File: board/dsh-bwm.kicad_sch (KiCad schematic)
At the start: 15 parts, among them IC2 MAX485CSA+T, K1 833H-1C-C-24VDC, K2 833H-1C-C-24VDC, K3 833H-1C-C-24VDC, K4 833H-1C-C-24VDC, Q1 IRLB8721PBF, U1 Pico

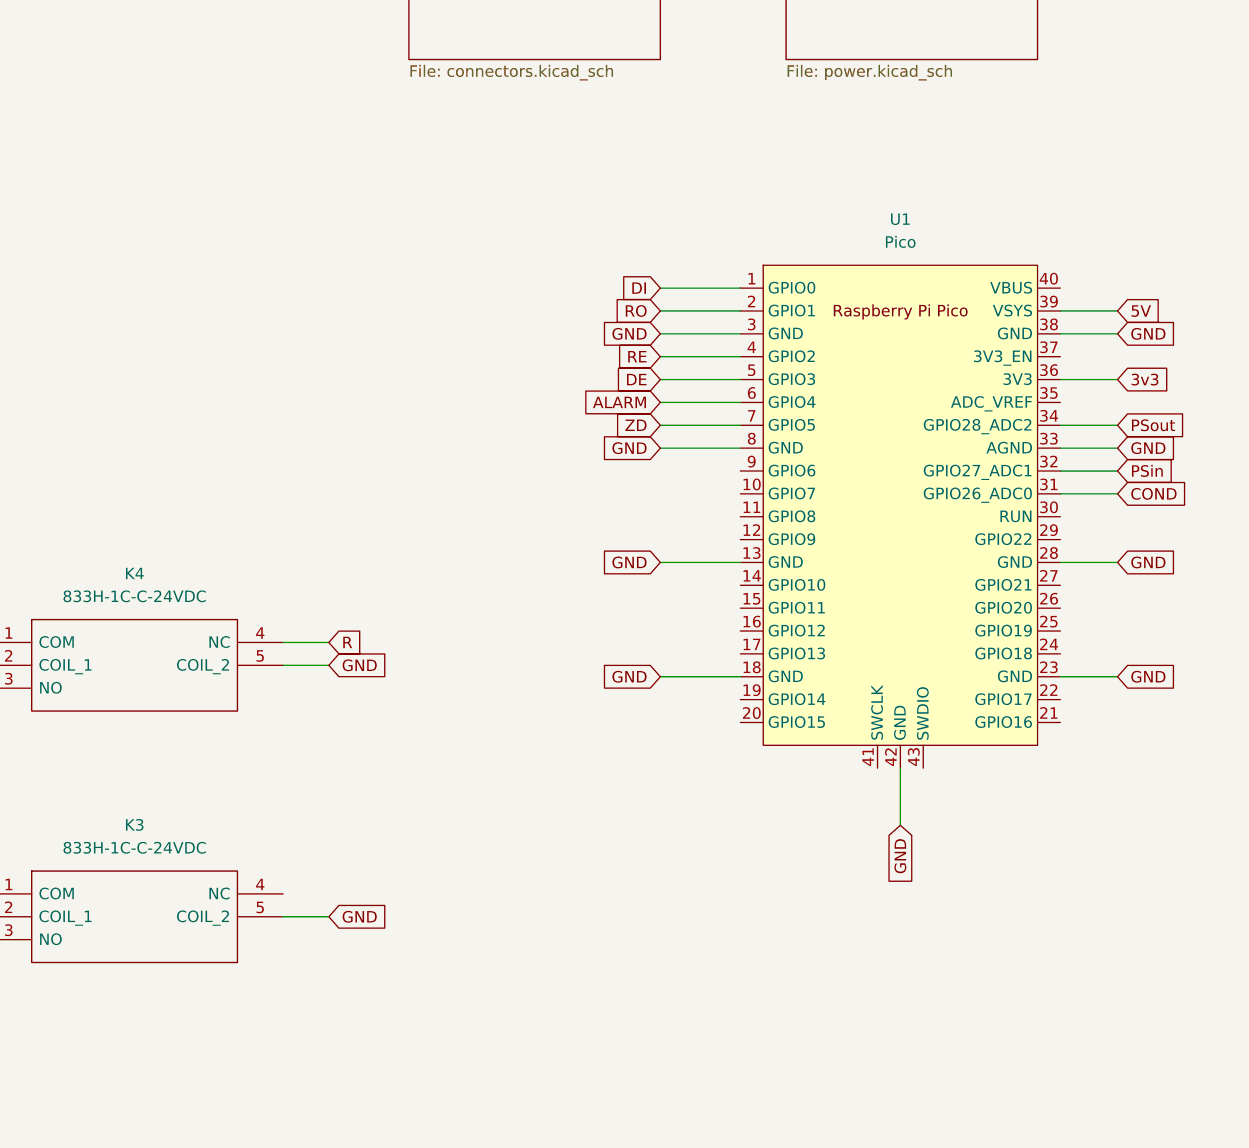
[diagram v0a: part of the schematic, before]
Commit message: RP2040 Stamp
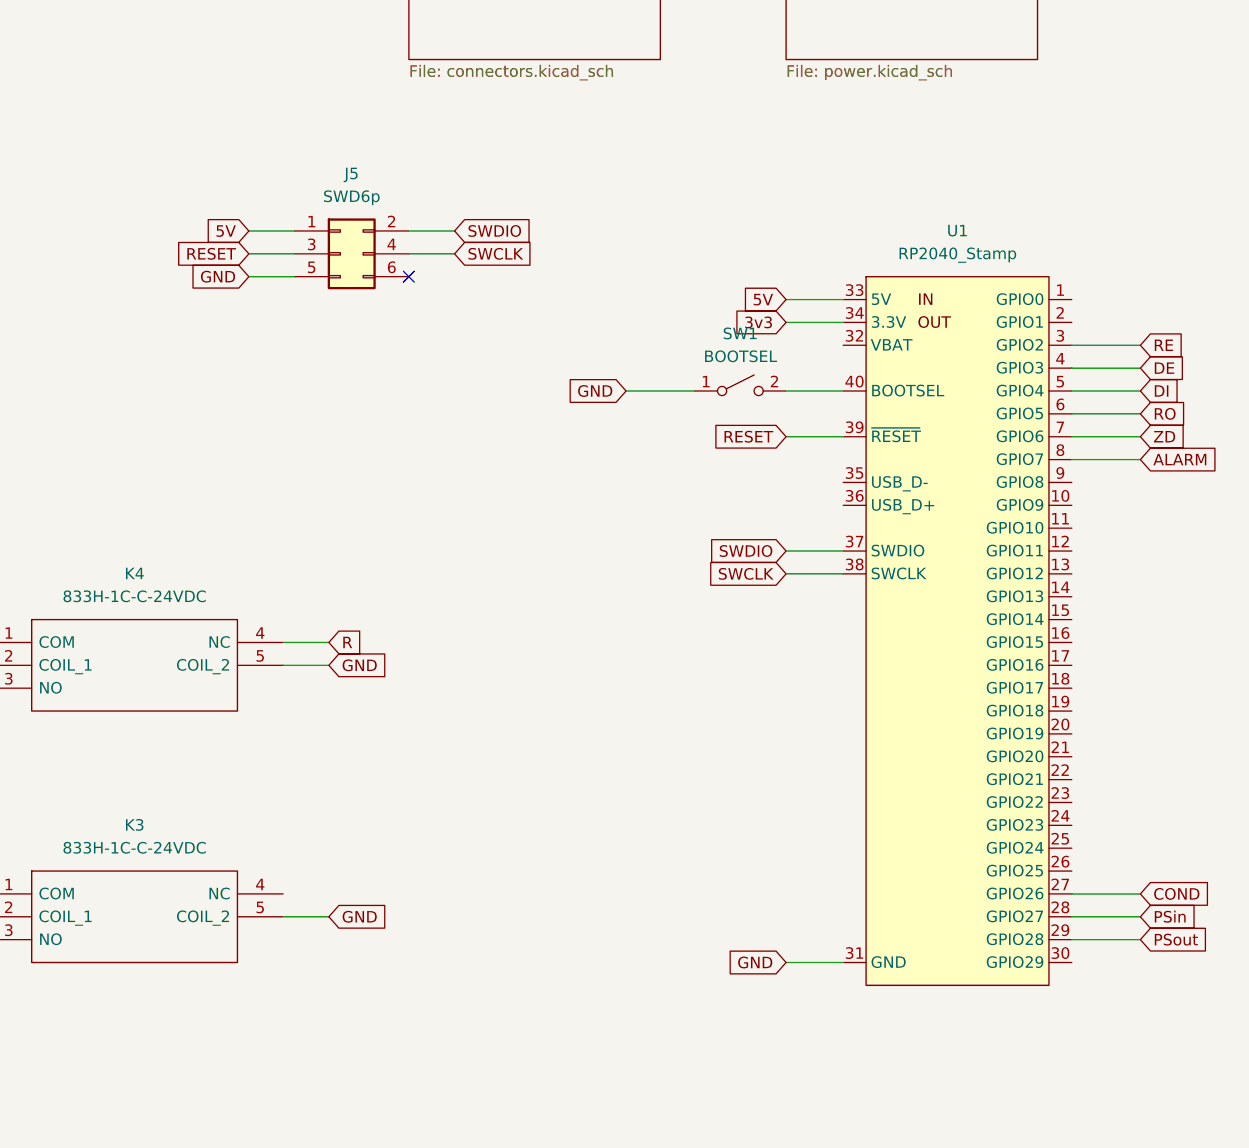
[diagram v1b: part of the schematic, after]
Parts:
- removed U1: Pico, MCU_RaspberryPi_and_Boards:RPi_Pico_SMD_TH, symbol MCU_RaspberryPi_and_Boards:Pico
- added J5: SWD6p, symbol Connector_Generic:Conn_02x03_Odd_Even
- added SW1: BOOTSEL, Button_Switch_SMD:SW_SPST_B3U-1000P, symbol Switch:SW_SPST
- added U1: RP2040_Stamp, SamacSys_Parts:RP2040_Stamp_SMD, symbol RP2040_Stamp:RP2040_Stamp
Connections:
- net 3v3: now also U1.34 (3.3V)
- net 5V: now also J5.1 (Pin_1), U1.33 (5V)
- net ALARM: now also U1.8 (GPIO7)
- net COND: now also U1.27 (GPIO26)
- net DE: now also U1.4 (GPIO3)
- net DI: now also U1.5 (GPIO4)
- net GND: now also J5.5 (Pin_5), SW1.1 (A), U1.31 (GND)
- net PSin: now also U1.28 (GPIO27)
- net PSout: now also U1.29 (GPIO28)
- net RE: now also U1.3 (GPIO2)
- net RO: now also U1.6 (GPIO5)
- net ZD: now also U1.7 (GPIO6)
- new net: SW1.2 (B), U1.40 (BOOTSEL)
- new net RESET: J5.3 (Pin_3), U1.39 (~{RESET})
- new net SWCLK: J5.4 (Pin_4), U1.38 (SWCLK)
- new net SWDIO: J5.2 (Pin_2), U1.37 (SWDIO)
- no-connect marks 0 -> 1

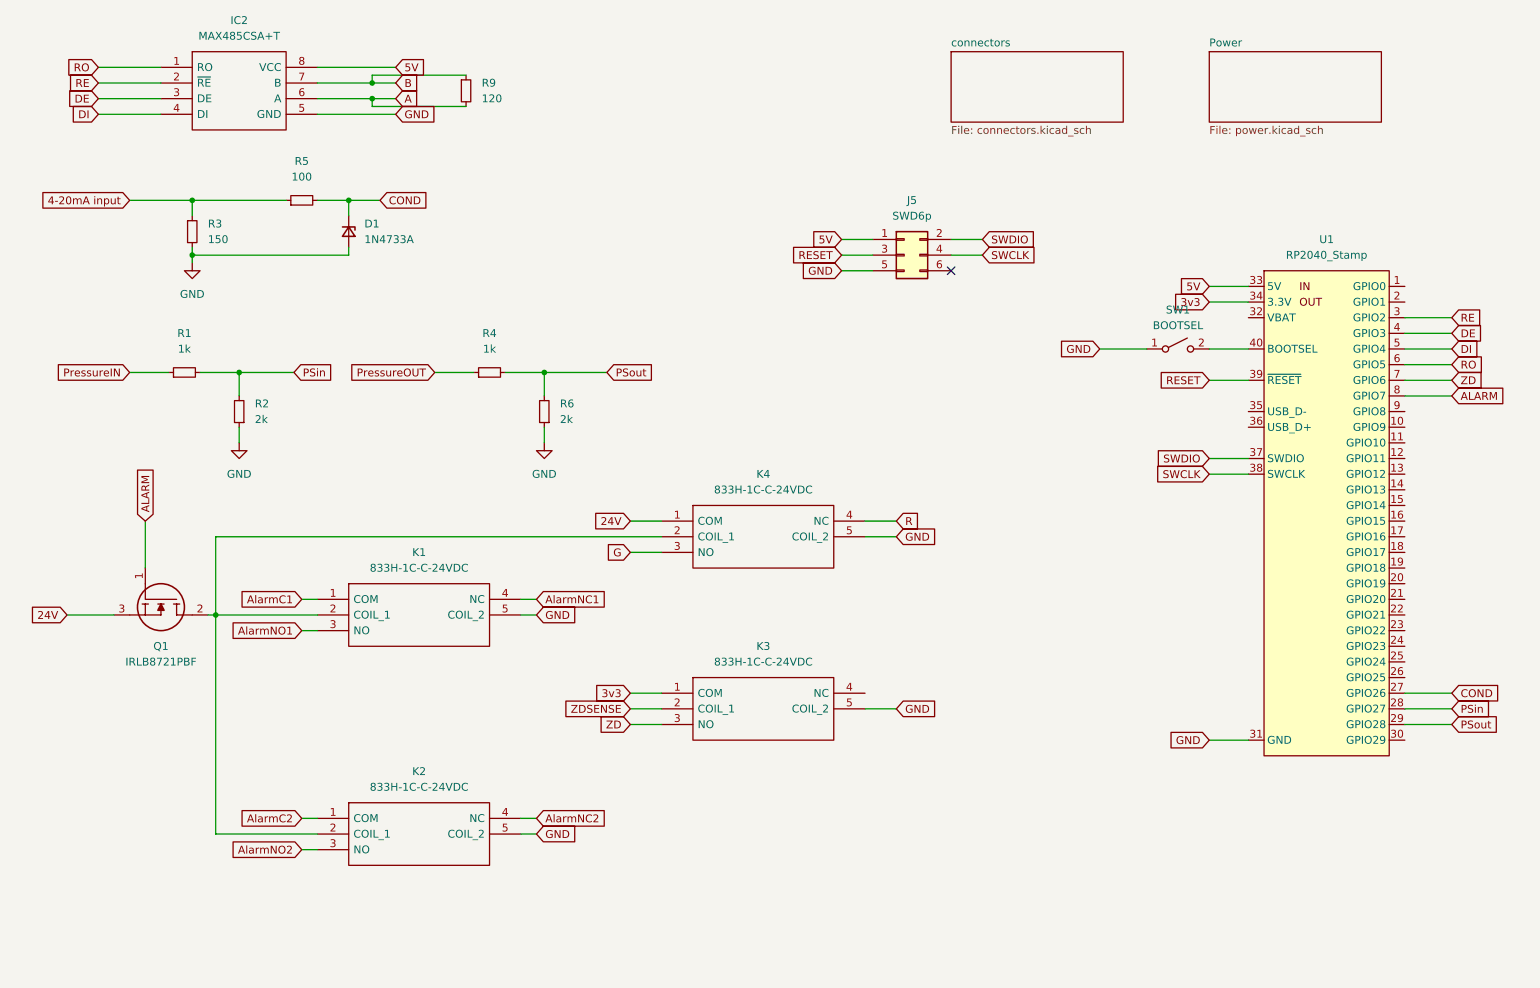
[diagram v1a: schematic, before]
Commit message: Power shit and copper fillz boi
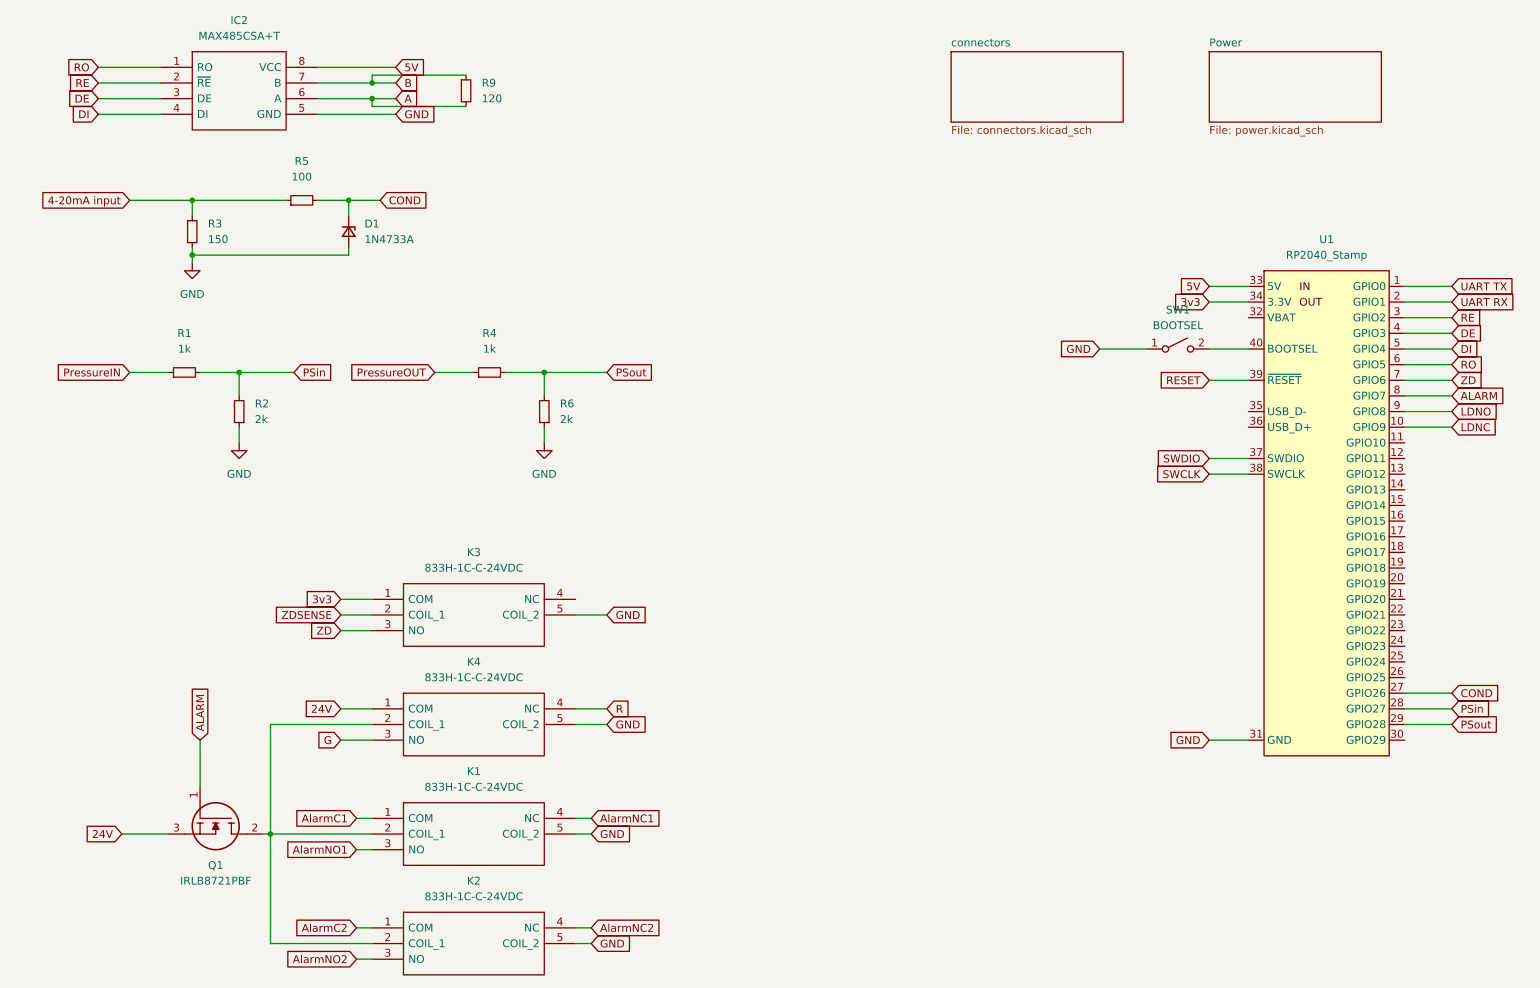
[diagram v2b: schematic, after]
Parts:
- removed J5: SWD6p, symbol Connector_Generic:Conn_02x03_Odd_Even
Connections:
- net UART TX: now reaches U1.1 (GPIO0)
- net LDNC: now reaches U1.10 (GPIO9)
- net UART RX: now reaches U1.2 (GPIO1)
- net LDNO: now reaches U1.9 (GPIO8)
- no-connect marks 1 -> 0
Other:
- moved on the sheet: K1, K2, K3, K4, Q1
